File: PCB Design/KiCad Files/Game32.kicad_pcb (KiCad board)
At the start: 2 copper layers, 20 parts, among them SW1 UP, SW2 DOWN, SW3 LEFT, SW4 RIGHT, SW5 SELECT, SW6 START, SW7 A, SW8 KEY, SW9 B, U1 ESP32-WROOM-32

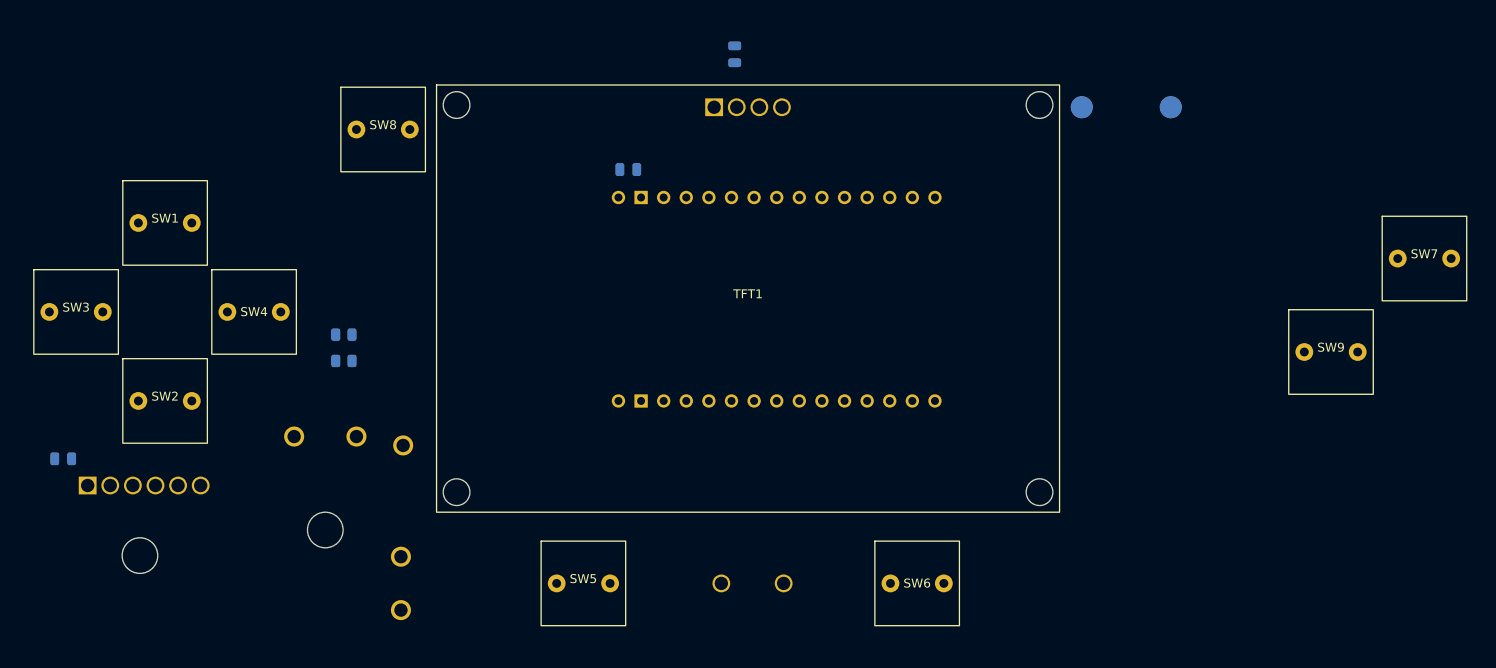
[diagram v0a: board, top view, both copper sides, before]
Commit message: PCB Completed
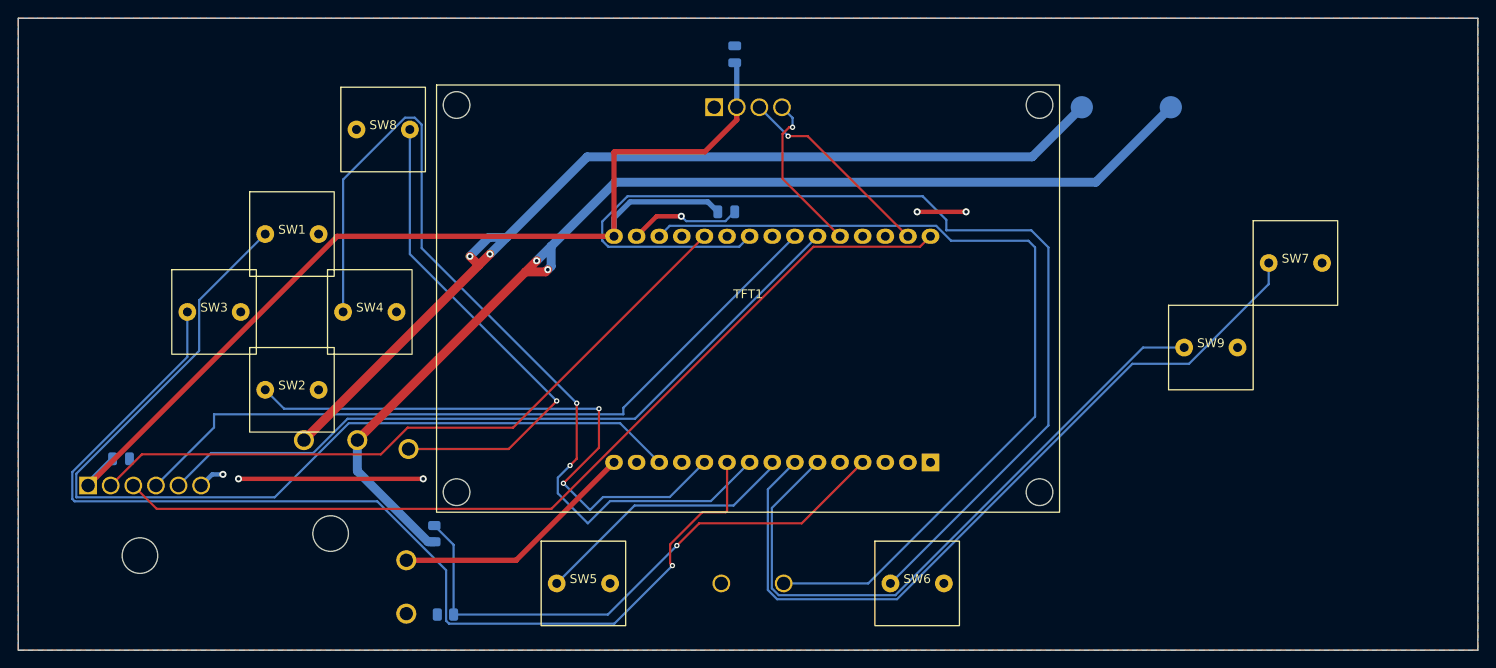
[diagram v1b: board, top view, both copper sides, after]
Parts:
- removed U1: ESP32-WROOM-32, RF_Module:ESP32-C3-DevKit-ELEGOO
- added ELEGOO_ESP1: ~, Custom Devkits:ELEGOO ESP32 DevKit Type C V1, B.Cu at (173.0, 106.4)
- C1, C2, C3: value C -> 103p
- R1, R2: value R -> 100k
- moved R2 30.7 mm to (112.5, 122.0), turned to 0 degrees
- moved R1 24.6 mm to (111.2, 112.9), turned to -90 degrees
- moved PD1 16.0 mm to (89.6, 125.9)
- moved SW3 15.5 mm to (86.5, 88.0)
- moved SW7 14.5 mm to (208.0, 82.5)
- moved SW1 14.3 mm to (95.2, 79.2)
- moved SW2 14.3 mm to (95.2, 96.8)
- moved SW9 13.5 mm to (198.5, 92.0)
- moved SW4 13.0 mm to (104.0, 88.0)
- moved C1 12.0 mm to (144.1, 76.8)
- moved C2 6.50 mm to (76.0, 104.5), turned to 0 degrees
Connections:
- C1 pad 1: Net-(SD_READER1-3V3) -> GND
- C1 pad 2: GND -> Net-(ELEGOO_ESP1-3V3)
- C2 pad 1: Net-(SD_READER1-3V3) -> Net-(ELEGOO_ESP1-3V3)
- C3 pad 1: Net-(SD_READER1-3V3) -> Net-(ELEGOO_ESP1-3V3)
- SD_READER1 pad 1: Net-(SD_READER1-3V3) -> Net-(ELEGOO_ESP1-3V3)
- TFT1 pad 1: Net-(SD_READER1-3V3) -> Net-(ELEGOO_ESP1-3V3)
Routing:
- net Net-(BT1-+): track 0.00 -> 127.7 mm, vias 0 -> 2
- net Net-(ELEGOO_ESP1-D27): track 0.00 -> 121.5 mm, vias 0 -> 1
- net Net-(ELEGOO_ESP1-3V3): track 0.00 -> 121.3 mm
- net Net-(ELEGOO_ESP1-TX2/D17): track 0.00 -> 119.0 mm
- net Net-(BT1--): track 0.00 -> 109.3 mm, vias 0 -> 2
- net Net-(ELEGOO_ESP1-D13): track 0.00 -> 109.1 mm
- net Net-(ELEGOO_ESP1-D23): track 0.00 -> 103.3 mm
- net Net-(ELEGOO_ESP1-D26): track 0.00 -> 102.2 mm, vias 0 -> 2
- net Net-(BZ1-+): track 0.00 -> 98.7 mm
- net Net-(ELEGOO_ESP1-D33): track 0.00 -> 89.3 mm
- net Net-(ELEGOO_ESP1-D18): track 0.00 -> 85.0 mm
- net Net-(ELEGOO_ESP1-D19): track 0.00 -> 83.6 mm
- net Net-(ELEGOO_ESP1-D4): track 0.00 -> 78.3 mm
- net Net-(ELEGOO_ESP1-D32): track 0.00 -> 74.4 mm
- net Net-(ELEGOO_ESP1-D14): track 0.00 -> 67.7 mm, vias 0 -> 2
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- added copper zone on B.Cu, net GND
- added copper zone on F.Cu, net GND
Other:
- board outline added: 164 x 71 mm
